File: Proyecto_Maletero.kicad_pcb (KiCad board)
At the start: 2 copper layers, 74.8 x 59.6 mm, 43 parts, among them J1 DE9_Pins, J2 Conn_01x02, J3 Conn_01x02, J4 Conn_01x03, J5 Conn_01x02, J6 DE9_Pins, J8 Conn_01x02, J9 Conn_01x02, K1 FINDER-34.51, Q2 MMBT5550L, U1 LM1084-5.0, U2 MCP2551-I-SN, U3 PIC18F258-I_SO, U5 LM321, U6 LM1084-5.0, U7 DRV8870DDA, Y1 4MHz

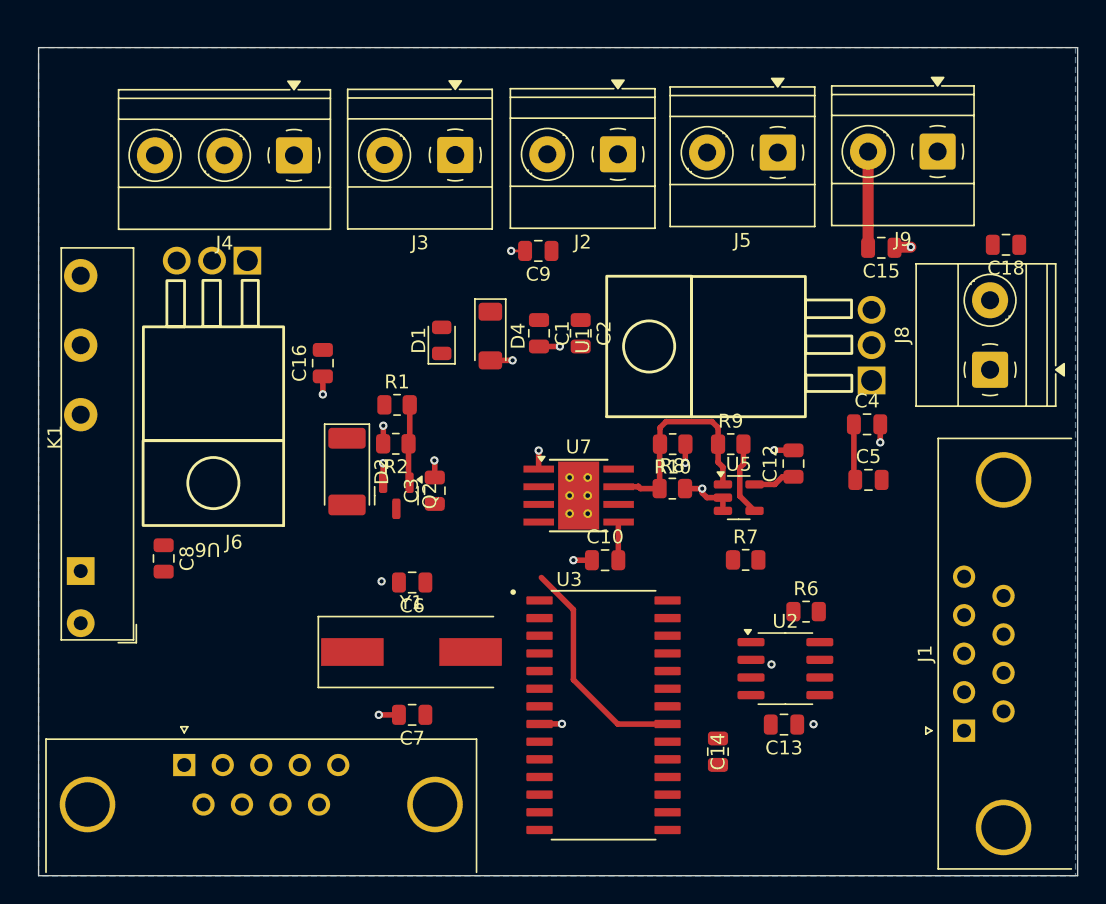
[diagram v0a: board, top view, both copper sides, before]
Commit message: Layout final v.1
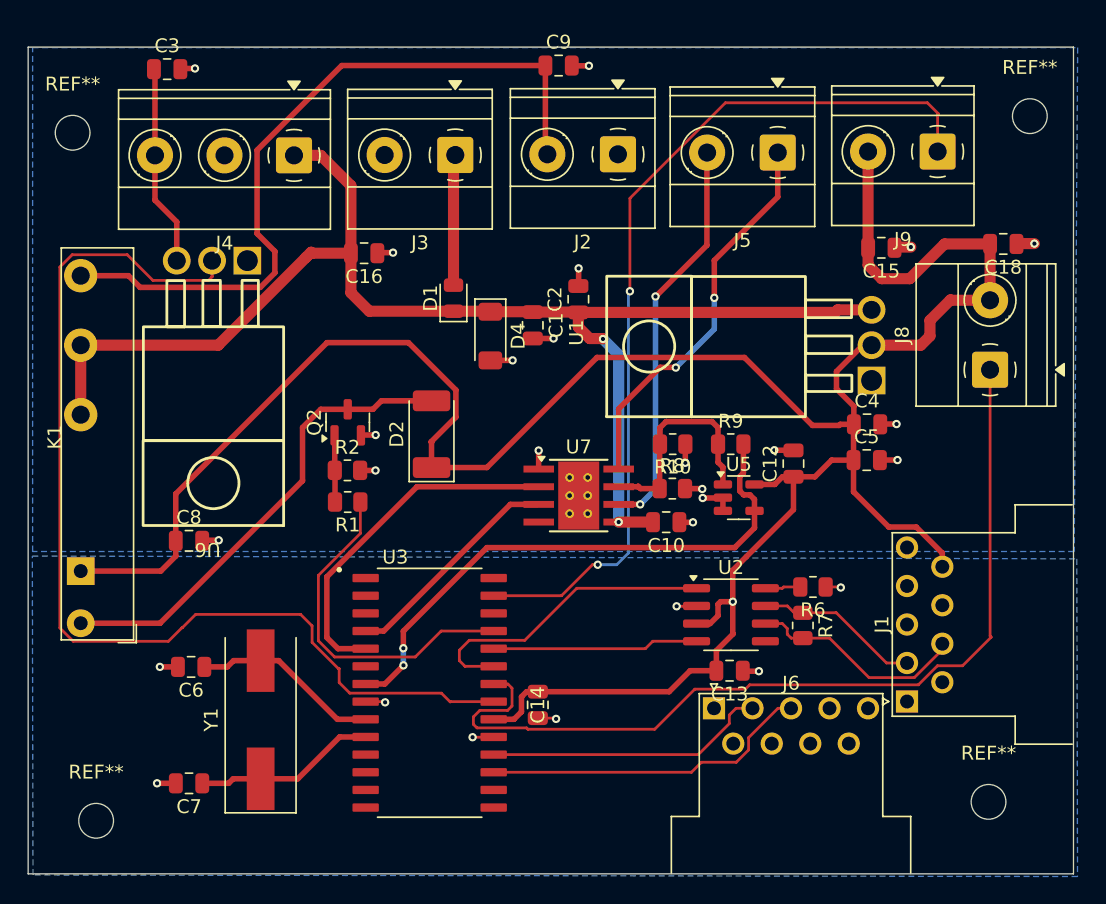
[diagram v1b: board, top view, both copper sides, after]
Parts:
- added REF**: MountingHole_2.5mm, MountingHole:MountingHole_2.5mm, F.Cu at (95.8, 76.8)
- added REF**: MountingHole_2.5mm, MountingHole:MountingHole_2.5mm, F.Cu at (29.9, 28.6)
- added REF**: MountingHole_2.5mm, MountingHole:MountingHole_2.5mm, F.Cu at (31.6, 78.1)
- added REF**: MountingHole_2.5mm, MountingHole:MountingHole_2.5mm, F.Cu at (98.8, 27.4)
- J1, J6: footprint Connector_Dsub:DSUB-9_Pins_Horizontal_P2.77x2.84mm_EdgePinOffset4.94mm_Housed_MountingHolesOffset4.94mm -> Connector_Dsub:DSUB-9_Pins_Horizontal_P2.77x2.54mm_EdgePinOffset9.40mm
- moved J6 38.3 mm to (76.1, 70.0)
- moved C3 35.9 mm to (36.8, 24.1), turned to 0 degrees
- moved C6 17.0 mm to (38.5, 67.0)
- moved C7 16.8 mm to (38.3, 75.4)
- moved C9 13.4 mm to (64.9, 23.8), turned to 0 degrees
- moved C14 13.4 mm to (63.4, 69.8)
- moved U3 12.6 mm to (55.6, 68.9)
- moved Y1 11.9 mm to (43.5, 70.8), turned to 90 degrees
- moved C16 8.45 mm to (50.9, 37.3), turned to 180 degrees
- moved R1 7.84 mm to (49.7, 55.2), turned to 180 degrees
- moved D2 6.65 mm to (55.8, 50.3), turned to 90 degrees
- moved Q2 6.33 mm to (49.7, 49.5), turned to 90 degrees
- moved R7 6.26 mm to (82.5, 64.1), turned to -90 degrees
- moved C13 5.51 mm to (77.2, 67.3)
- moved U2 5.51 mm to (77.3, 63.3)
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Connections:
- C1 pad 2: GND -> GNDPWR
- C10 pad 1: GND -> GNDPWR
- C12 pad 2: GND -> GNDPWR
- C15 pad 1: GND -> GNDPWR
- C16 pad 1: GND -> GNDPWR
- C18 pad 1: GND -> GNDPWR
- C2 pad 2: GND -> GNDPWR
- C3 pad 2: GND -> GNDPWR
- C4 pad 2: GND -> GNDPWR
- C5 pad 2: GND -> GNDPWR
- C8 pad 2: GND -> GNDPWR
- C9 pad 2: GND -> GNDPWR
- D4 pad 2: GND -> GNDPWR
- J2 pad 1: GND -> GNDPWR
- J3 pad 2: GND -> GNDPWR
- J4 pad 2: GND -> GNDPWR
- Q2 pad 2: GND -> GNDPWR
- R10 pad 1: GND -> GNDPWR
- R2 pad 2: GND -> GNDPWR
- R8 pad 2: GND -> GNDPWR
- U1 pad 1: GND -> GNDPWR
- U5 pad 2: GND -> GNDPWR
- U5 pad 3: GND -> GNDPWR
- U6 pad 1: GND -> unconnected-(U6-GND-Pad1)
- U7 pad 1: GND -> GNDPWR
- U7 pad 9: GND -> GNDPWR
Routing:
- net VCC: track 14.1 -> 180.6 mm, vias 0 -> 1
- net VBAT: track 2.76 -> 97.4 mm, vias 0 -> 2
- net SENAL_RELE: track 0.00 -> 65.8 mm
- net Manual_Close: track 0.00 -> 64.6 mm, vias 0 -> 2
- net Sensor_Pie: track 16.4 -> 75.6 mm
- net VRth: track 0.09 -> 53.8 mm
- net Vopam: track 5.37 -> 41.0 mm, vias 0 -> 2
- net Net-(D2-A): track 0.00 -> 34.1 mm
- net Motor+: track 0.00 -> 28.9 mm, vias 0 -> 2
- net Motor-: track 0.00 -> 28.2 mm, vias 0 -> 2
- net PH_B: track 0.00 -> 25.4 mm
- net INPUT_RELE: track 0.00 -> 25.1 mm
- net GNDPWR: track 0.00 -> 24.9 mm, vias 0 -> 19
- net TX_USART: track 0.00 -> 23.8 mm
- net CAN_TX: track 0.00 -> 22.3 mm
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- added copper zone on B.Cu, net GNDPWR
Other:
- board size 74.8 x 59.6 mm -> 75.2 x 59.5 mm
